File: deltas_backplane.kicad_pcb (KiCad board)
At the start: 2 copper layers, 140.6 x 119.4 mm, 11 parts, among them J1 SNP_female_straight, J2 SNP_female_straight, J3 SNP_female_straight, J4 SNP_female_straight, J5 SNP_male_angle, J6 zx_bus, J7 zx_bus, J8 Barrel_Jack, SW1 SW_SPDT

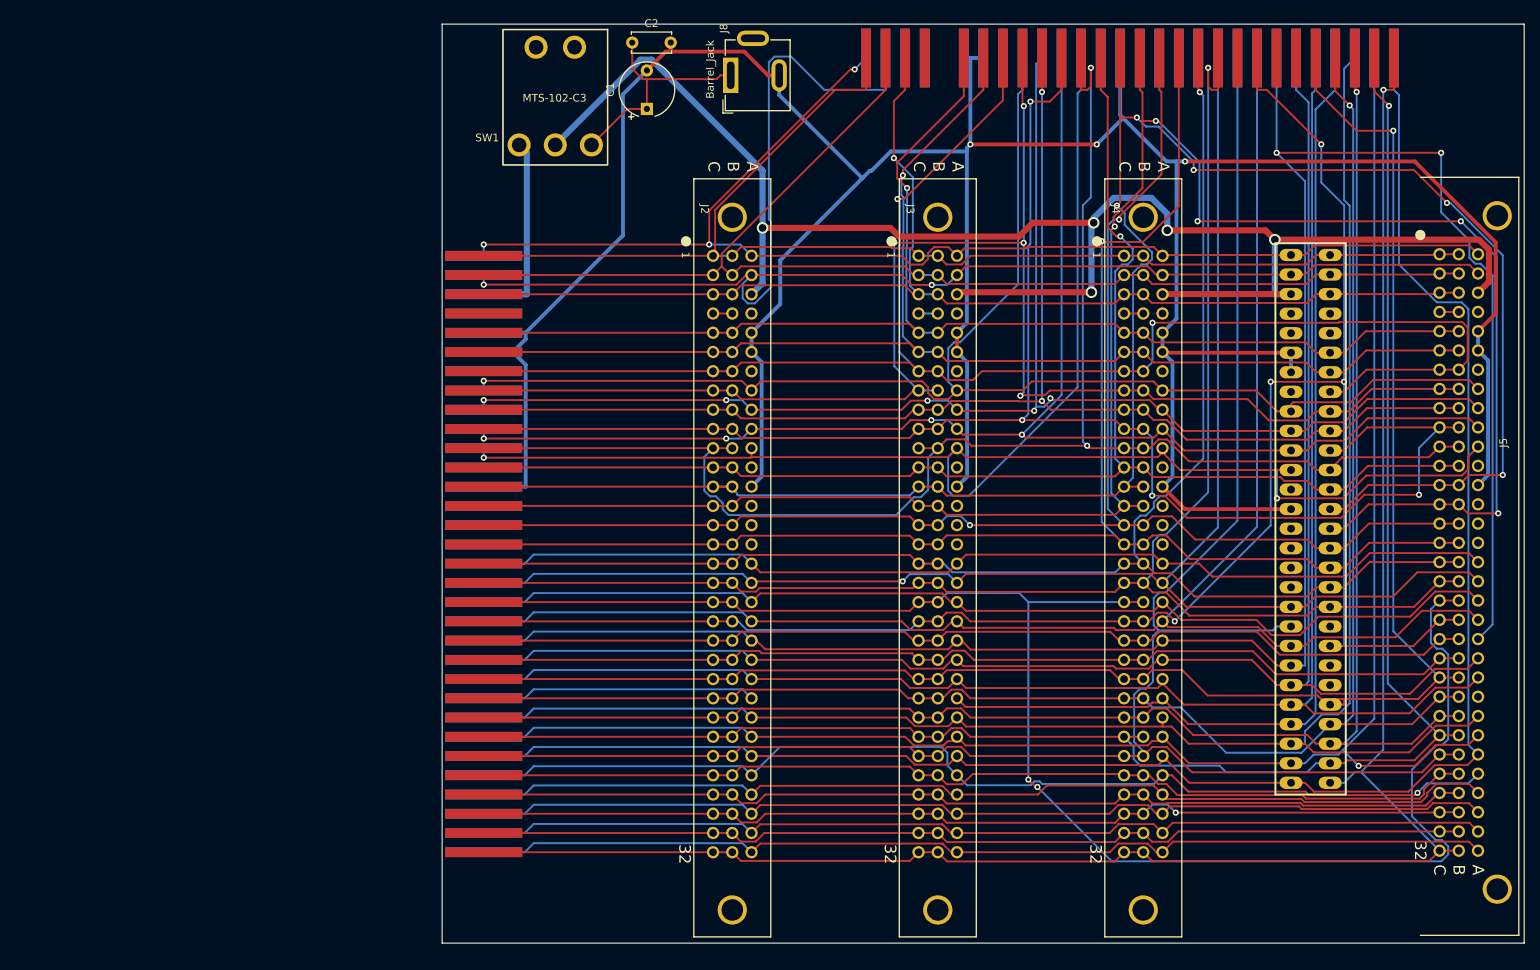
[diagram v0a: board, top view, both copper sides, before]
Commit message: 03.10.2023 update
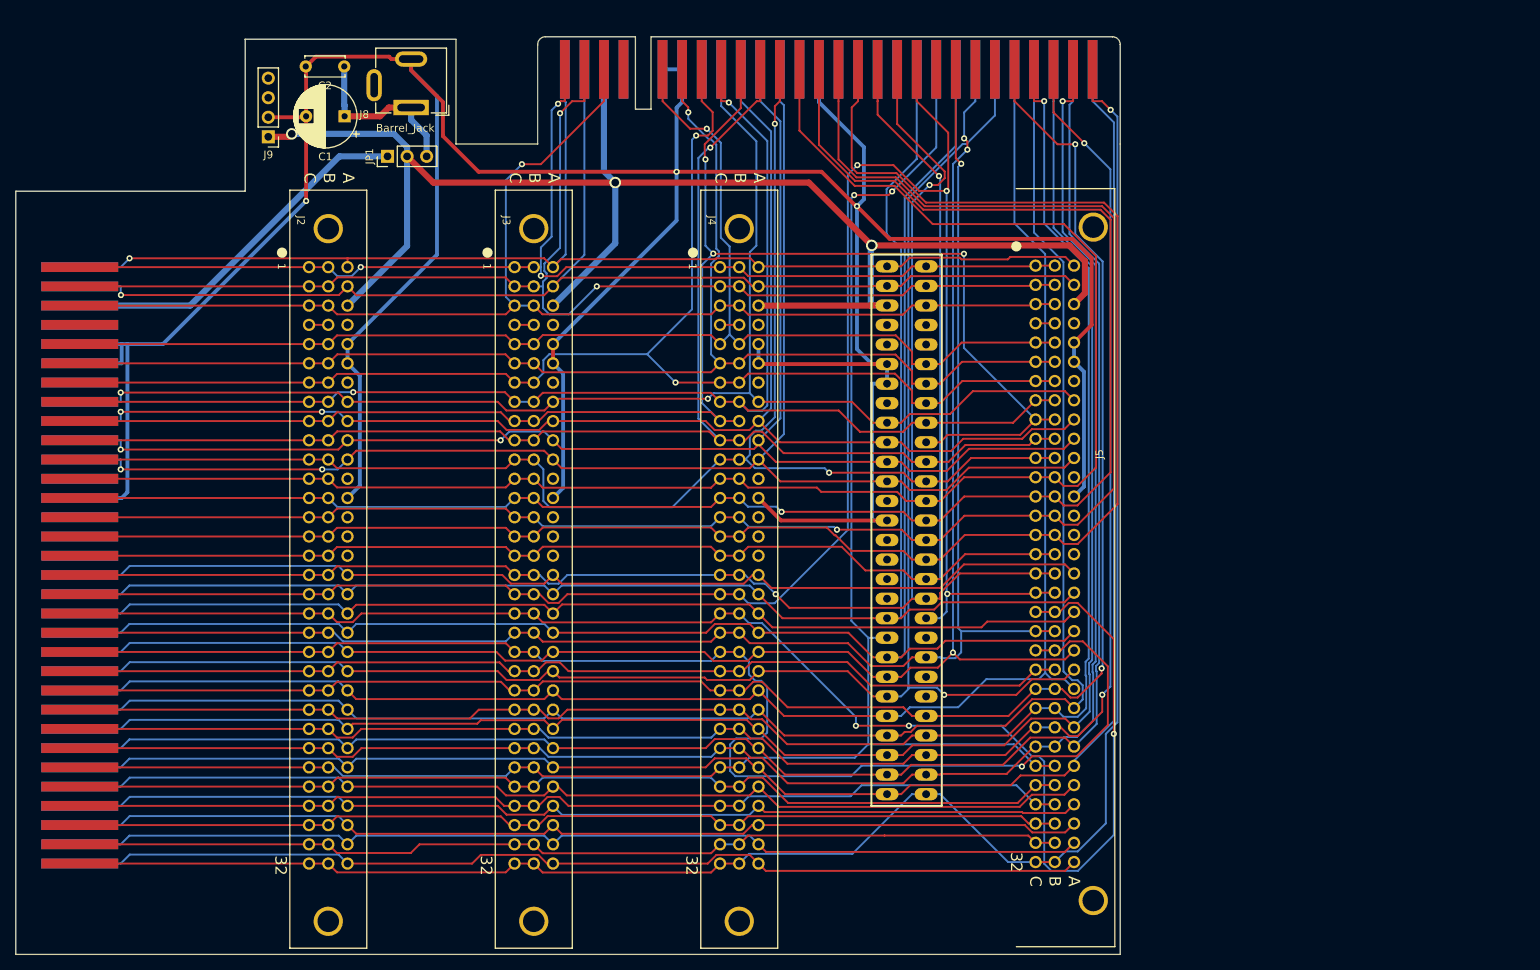
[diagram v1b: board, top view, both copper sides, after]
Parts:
- removed SW1: SW_SPDT, Backplane:MTS-102-C3
- added J9: Conn_01x04, Backplane_2:PinHeader_1x04_P2.54mm_Vertical, F.Cu at (118.0, 29.2)
- added JP1: Jumper_3_Open, Backplane_2:PinHeader_1x03_P2.54mm_Vertical, F.Cu at (133.5, 31.8)
- C1: footprint Capacitor_THT:CP_Radial_Tantal_D7.0mm_P5.00mm -> Backplane_2:CP_Radial_D8.0mm_P5.00mm
- C2: footprint Capacitor_THT:C_Disc_D5.0mm_W2.5mm_P5.00mm -> Backplane_2:C_Disc_D5.0mm_W2.5mm_P5.00mm
- J1: footprint Backplane:snp_straight -> Backplane_2:snp_straight
- J2, J3, J4: footprint Backplane:snp59_96_male_straight -> Backplane_2:snp59_96_male_straight
- J5: footprint Backplane:snp59_96_female_angle_3 -> Backplane_2:snp59_96_female_angle_3
- J6: footprint Backplane:ZX SPECTRUM EDGE CONNECTOR (HORIZONTAL) -> Backplane_2:ZX SPECTRUM EDGE CONNECTOR (HORIZONTAL)
- J7: footprint Backplane:Spectrum_edge_slot_FIXED -> Backplane_2:Spectrum_edge_slot_FIXED
- J8: footprint Backplane:BarrelJack_GCT_DCJ200-10-A_Horizontal -> Backplane_2:BarrelJack_GCT_DCJ200-10-A_Horizontal
- moved J2 52.5 mm to (128.3, 46.2)
- moved J3 52.5 mm to (155.0, 46.2)
- moved J7 52.5 mm to (200.9, 84.2)
- moved J1 52.5 mm to (98.5, 124.3)
- moved J4 52.5 mm to (181.7, 46.2)
- moved J5 52.5 mm to (222.7, 46.0)
- moved J8 41.7 mm to (136.6, 25.4), turned to 180 degrees
- moved C1 39.3 mm to (127.9, 26.6), turned to 180 degrees
- moved J6 39.2 mm to (190.8, 20.7)
- moved C2 37.6 mm to (127.9, 20.1), turned to 180 degrees
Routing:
- net A6: track 279.9 -> 212.9 mm, vias 2 -> 3
- net ЧТПЗУL: track 171.6 -> 222.4 mm
- net B21_SNP: track 131.2 -> 180.0 mm, vias 0 -> 1
- net ЗПL: track 211.1 -> 256.4 mm, vias 1 -> 3
- net GND: track 436.5 -> 479.3 mm
- net D5: track 176.5 -> 213.2 mm, vias 2 -> 3
- net СТОПL: track 263.7 -> 227.1 mm, vias 5 -> 1
- net НПРL: track 260.4 -> 225.2 mm, vias 5 -> 1
- net ОЗУL: track 197.1 -> 230.6 mm, vias 2 -> 0
- net ОЖИДL: track 240.3 -> 207.6 mm, vias 4 -> 1
- net ПРL: track 188.1 -> 218.6 mm, vias 1 -> 0
- net D2: track 207.6 -> 177.9 mm
- net A12: track 193.0 -> 163.6 mm, vias 2 -> 1
- net A3: track 217.3 -> 188.6 mm
- net D3: track 212.3 -> 185.0 mm, vias 4 -> 1
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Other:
- board size 140.6 x 119.4 mm -> 143.5 x 119.2 mm
